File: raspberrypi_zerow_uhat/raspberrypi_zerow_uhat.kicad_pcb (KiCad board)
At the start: 2 copper layers, 65 x 30 mm, 5 parts, among them J1 GPIO_CONNECTOR

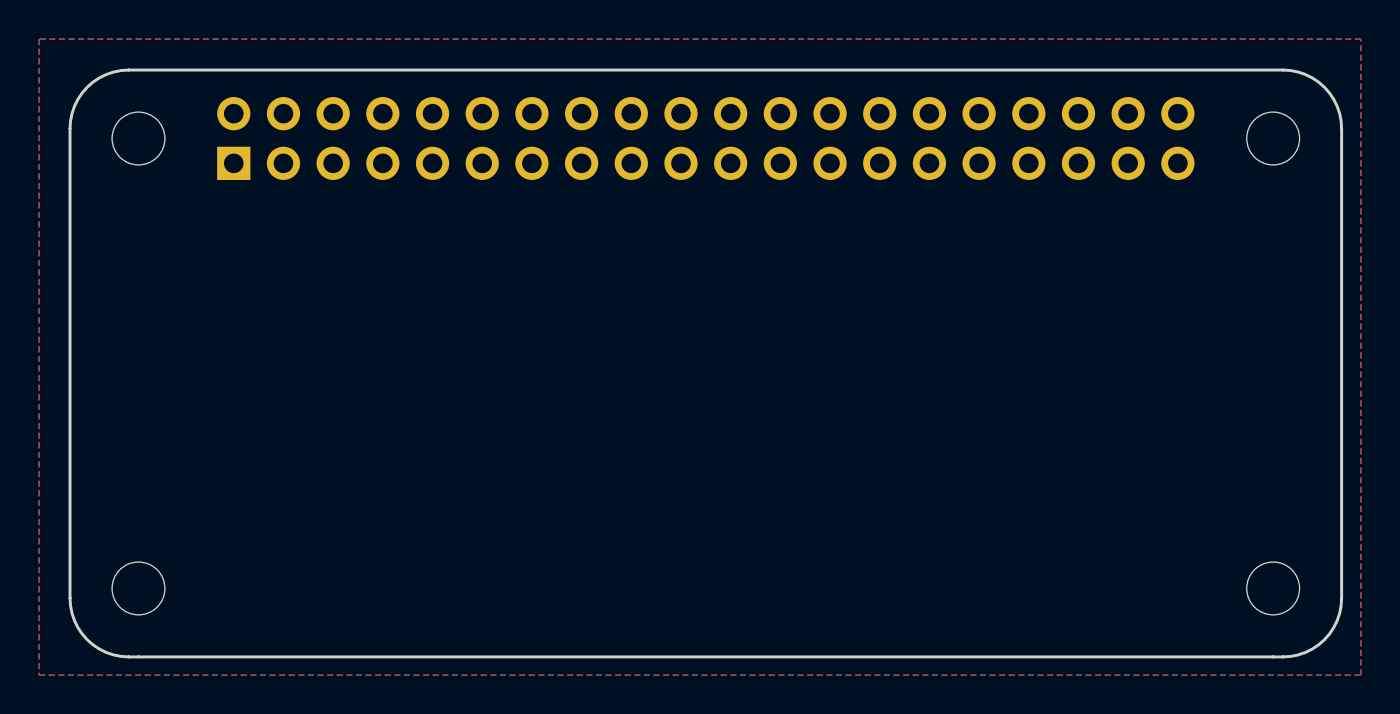
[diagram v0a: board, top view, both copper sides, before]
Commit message: work-in-progress
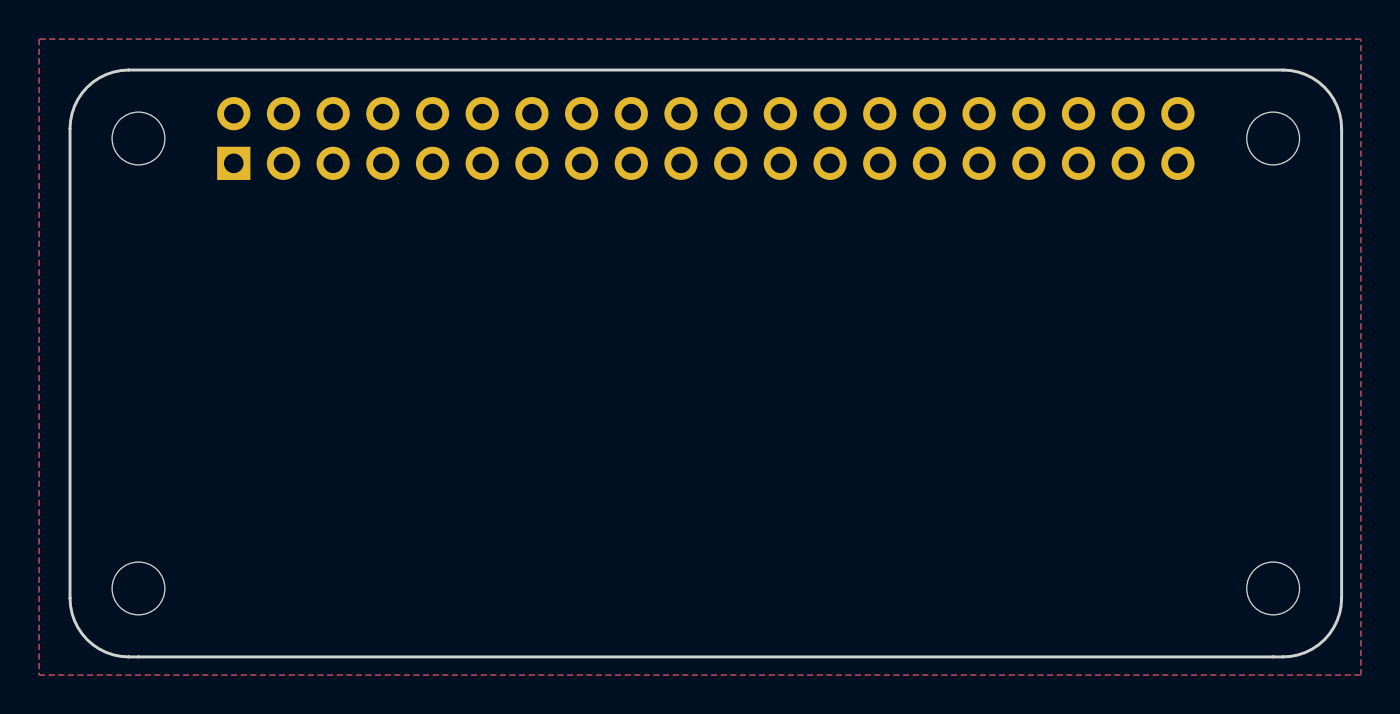
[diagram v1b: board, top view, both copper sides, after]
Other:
- net class Default removed
